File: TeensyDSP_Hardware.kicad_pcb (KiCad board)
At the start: 2 copper layers, 65 x 55 mm, 14 parts, among them J1 AudioJack2, U1 DM-OLED096-636, U2 TL072, U5 Teensy4.0

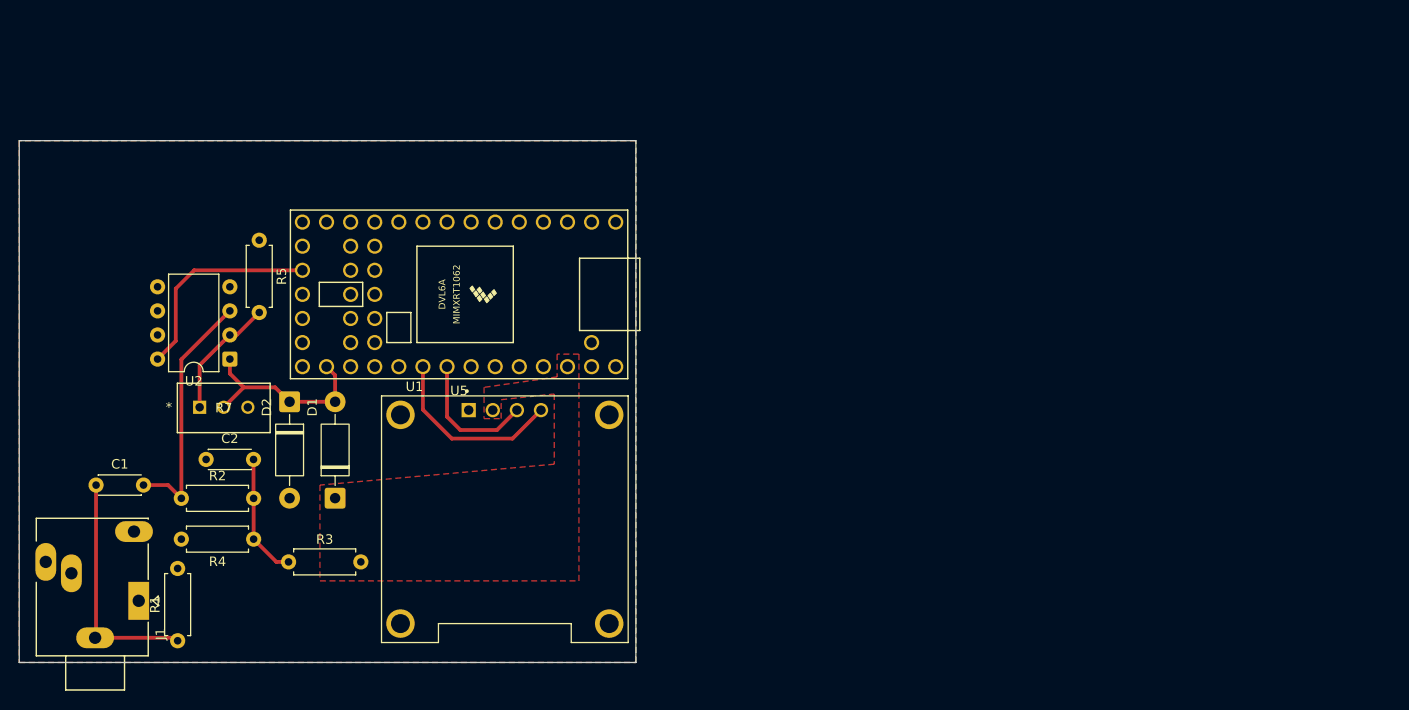
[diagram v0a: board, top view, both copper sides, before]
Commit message: move toward guitar tuner
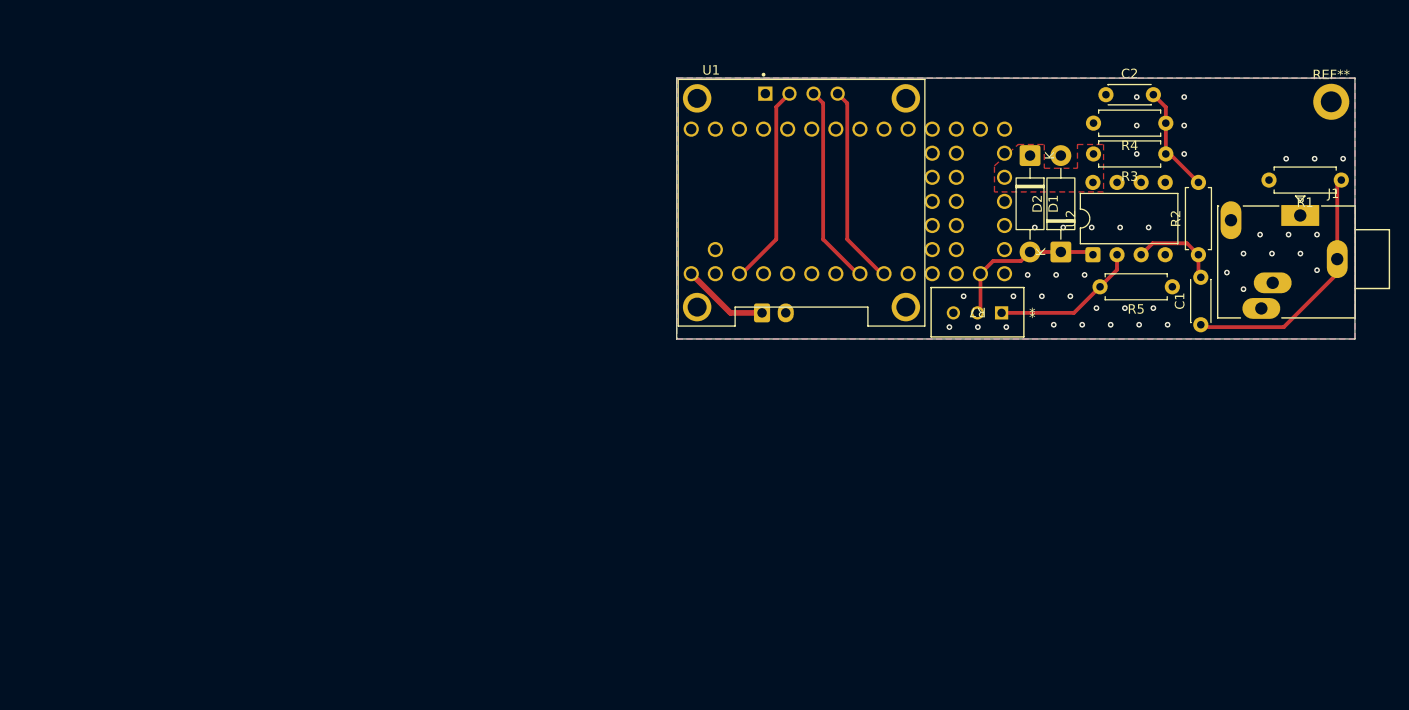
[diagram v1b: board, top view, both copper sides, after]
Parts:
- added J2: Conn_01x02_Socket, Connector_JST:JST_EH_B2B-EH-A_1x02_P2.50mm_Vertical, B.Cu at (127.5, 75.8)
- added REF**: MountingHole_2.2mm_M2_DIN965_Pad, MountingHole:MountingHole_2.2mm_M2_DIN965_Pad, F.Cu at (187.5, 53.5)
- U5: moved to B.Cu
- moved R1 131.9 mm to (188.6, 61.8), turned to 180 degrees
- moved J1 129.0 mm to (184.2, 65.5), turned to 180 degrees
- moved C1 117.7 mm to (173.8, 77.0), turned to 90 degrees
- moved R2 110.2 mm to (173.5, 69.6), turned to 90 degrees
- moved R4 105.7 mm to (170.1, 55.8)
- moved C2 102.3 mm to (163.8, 52.8)
- moved R3 102.0 mm to (170.1, 59.0), turned to 180 degrees
- moved R5 96.4 mm to (170.8, 73.0), turned to 180 degrees
- moved U2 91.6 mm to (162.4, 69.6), turned to 90 degrees
- moved R7 85.1 mm to (152.8, 75.8), turned to 180 degrees
- moved D2 82.8 mm to (159.0, 69.3), turned to 90 degrees
- moved D1 81.7 mm to (155.8, 59.2), turned to -90 degrees
- moved U1 45.7 mm to (131.7, 64.1)
- moved U5 42.1 mm to (136.6, 64.0), turned to 0 degrees
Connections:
- U5 pad 33: unconnected-(U5-VIN-Pad33) -> Net-(J2-Pin_1)
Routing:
- net Net-(U2A-+): track 26.4 -> 9.77 mm
- net Net-(J2-Pin_1): track 0.00 -> 9.17 mm
- net /SCL: track 14.1 -> 21.3 mm
- net /A0: track 20.9 -> 17.2 mm
- net Net-(U2A--): track 13.0 -> 15.6 mm
- net Net-(C1-Pad1): track 25.0 -> 26.8 mm
- net /SDA: track 19.5 -> 21.3 mm
- net Net-(C2-Pad2): track 13.1 -> 11.5 mm
- net +3V3: track 22.4 -> 21.4 mm
- net GND: vias 0 -> 41
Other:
- board size 65 x 55 mm -> 71.5 x 27.5 mm

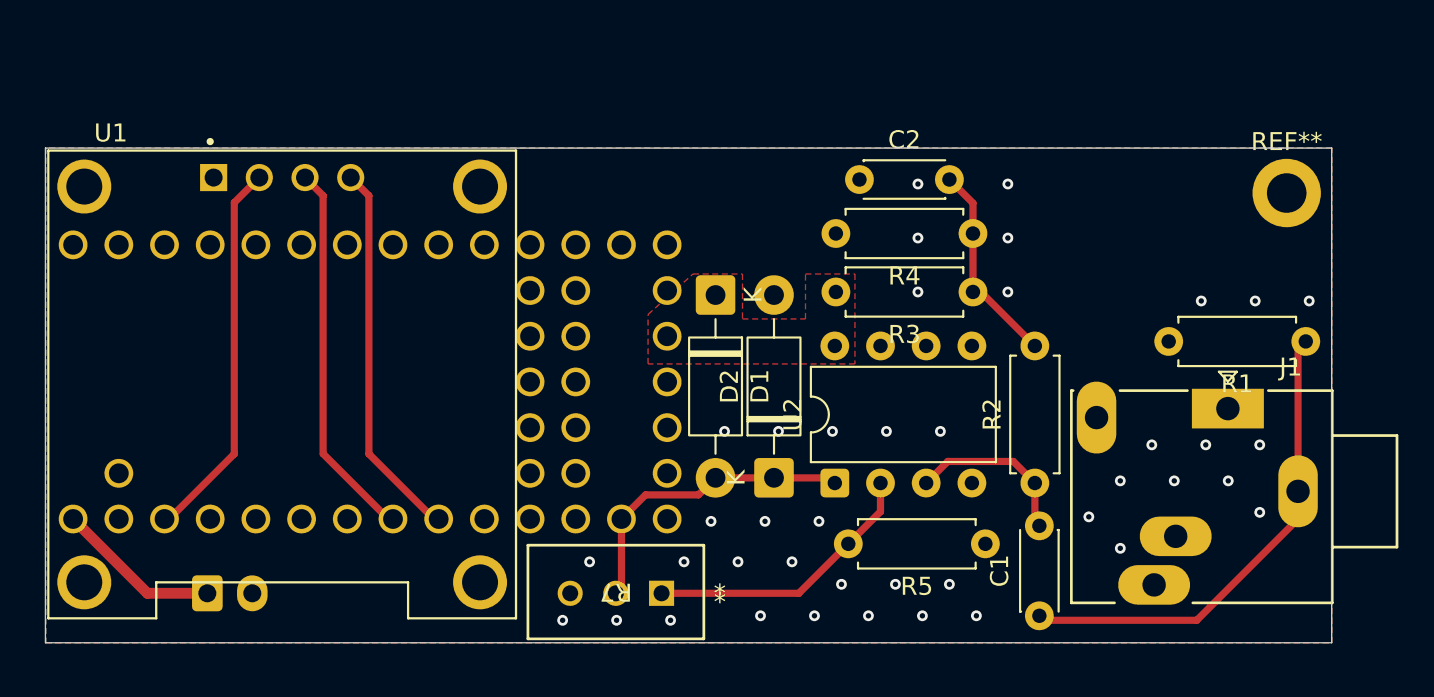
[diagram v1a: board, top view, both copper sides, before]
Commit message: Ordered Guitar Tuner
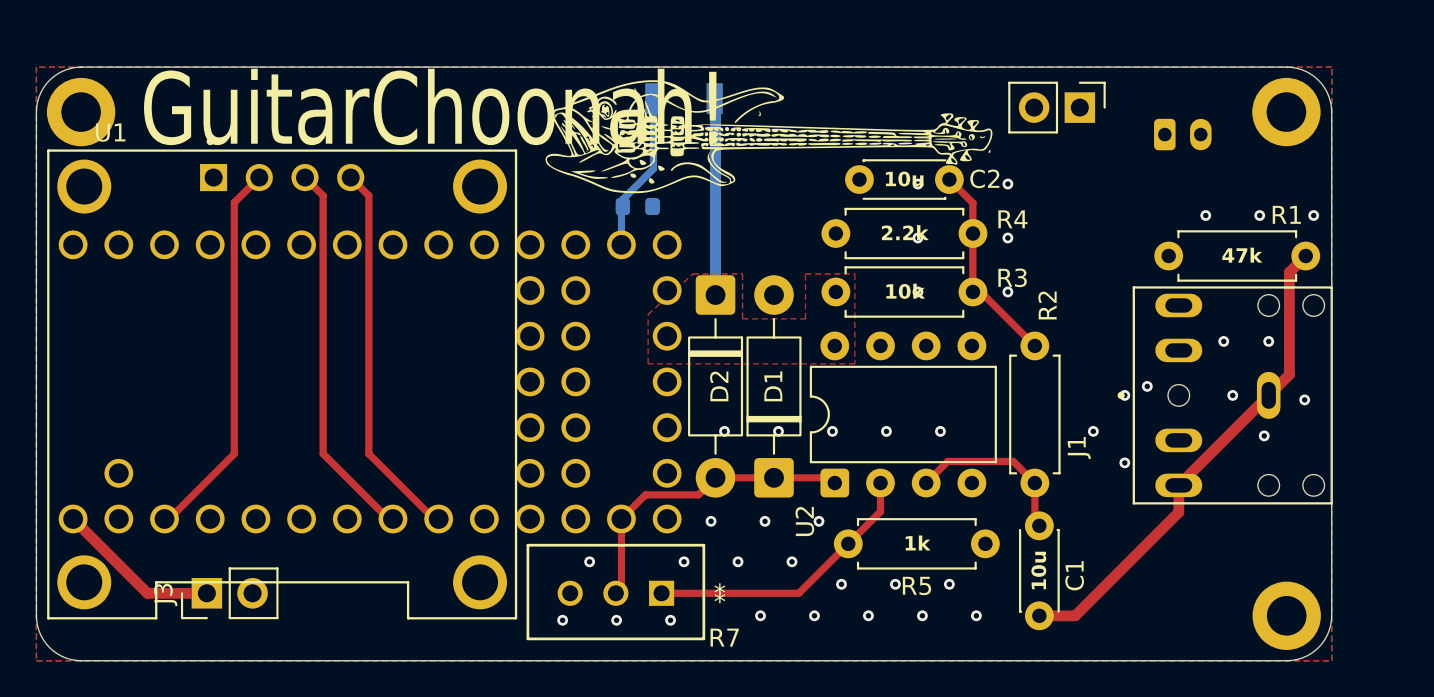
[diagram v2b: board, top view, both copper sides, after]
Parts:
- added J3: ChargerBoard, Connector_PinHeader_2.54mm:PinHeader_1x02_P2.54mm_Vertical, F.Cu at (127.5, 75.8)
- added J4: BatteryConnector, Connector_PinHeader_2.54mm:PinHeader_1x02_P2.54mm_Vertical, F.Cu at (176.0, 48.8)
- added R6: 10k, Resistor_SMD:R_0603_1608Metric, B.Cu at (151.4, 54.2)
- added REF**: MountingHole_2.2mm_M2_DIN965_Pad, MountingHole:MountingHole_2.2mm_M2_DIN965_Pad, F.Cu at (187.5, 77.0)
- added REF**: MountingHole_2.2mm_M2_DIN965_Pad, MountingHole:MountingHole_2.2mm_M2_DIN965_Pad, F.Cu at (120.5, 49.0)
- added SW1: SW_Push, Button_Switch_SMD:SW_SPST_B3U-3000P, B.Cu at (154.0, 48.2)
- J1: value AudioJack2 -> SJ1-3525N; footprint Connector_Audio:Jack_3.5mm_Ledino_KB3SPRS_Horizontal -> MyComponents:CUI_SJ1-3525N
- J2: footprint Connector_JST:JST_EH_B2B-EH-A_1x02_P2.50mm_Vertical -> Connector_JST:JST_PH_B2B-PH-K_1x02_P2.00mm_Vertical
- moved J2 59.0 mm to (180.7, 50.2)
- moved R1 4.75 mm to (188.6, 57.0)
- moved REF** 4.50 mm to (187.5, 49.0)
- moved J1 2.39 mm to (186.5, 64.8), turned to 90 degrees
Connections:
- J2 pad 1: Net-(J2-Pin_1) -> +BATT
- U5 pad 13: unconnected-(U5-11_MOSI_CTX1-Pad13) -> Net-(U5-11_MOSI_CTX1)
- U5 pad 33: Net-(J2-Pin_1) -> Net-(J3-Pin_1)
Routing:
- net +3V3: track 21.4 -> 32.4 mm
- net Net-(J3-Pin_1): track 0.00 -> 9.17 mm
- net Net-(J2-Pin_1): track 9.17 -> 0.00 mm
- net Net-(U5-11_MOSI_CTX1): track 0.00 -> 8.87 mm
- net Net-(C1-Pad1): track 26.8 -> 27.3 mm
- net GND: vias 41 -> 42
- added copper zone on In1.Cu, net GND
- added copper zone on In2.Cu, net GND
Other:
- board size 71.5 x 27.5 mm -> 72 x 33 mm
- copper layers 2 -> 4
- board text added: "10k"
- board text added: "10u"
- board text added: "1k"
- board text added: "2.2k"
- board text added: "47k"
- board text added: "BATT"
- board text added: "GuitarChoonah!"
